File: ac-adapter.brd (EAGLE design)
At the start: 81.3 x 73.7 mm, 45 parts, among them IC2 TL431, Q1 300V5A, Q2 300V5A, Q3 TLP621-1, T1 COMMON_FILTER-SU10VFC, T2 TRANSFORMAER_FLYBACK-PQ2620, T3 COMMON_FILTER-SMALL

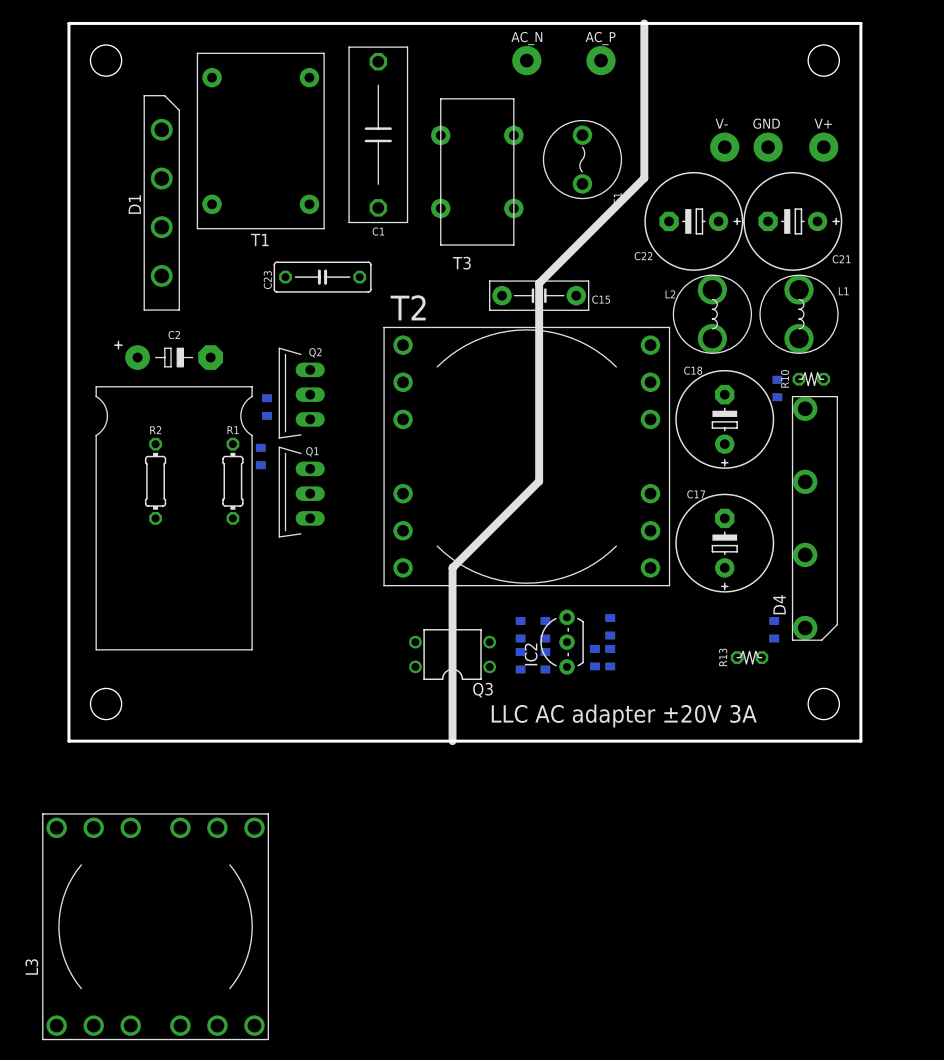
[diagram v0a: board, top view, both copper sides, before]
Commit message: 定数決まらん
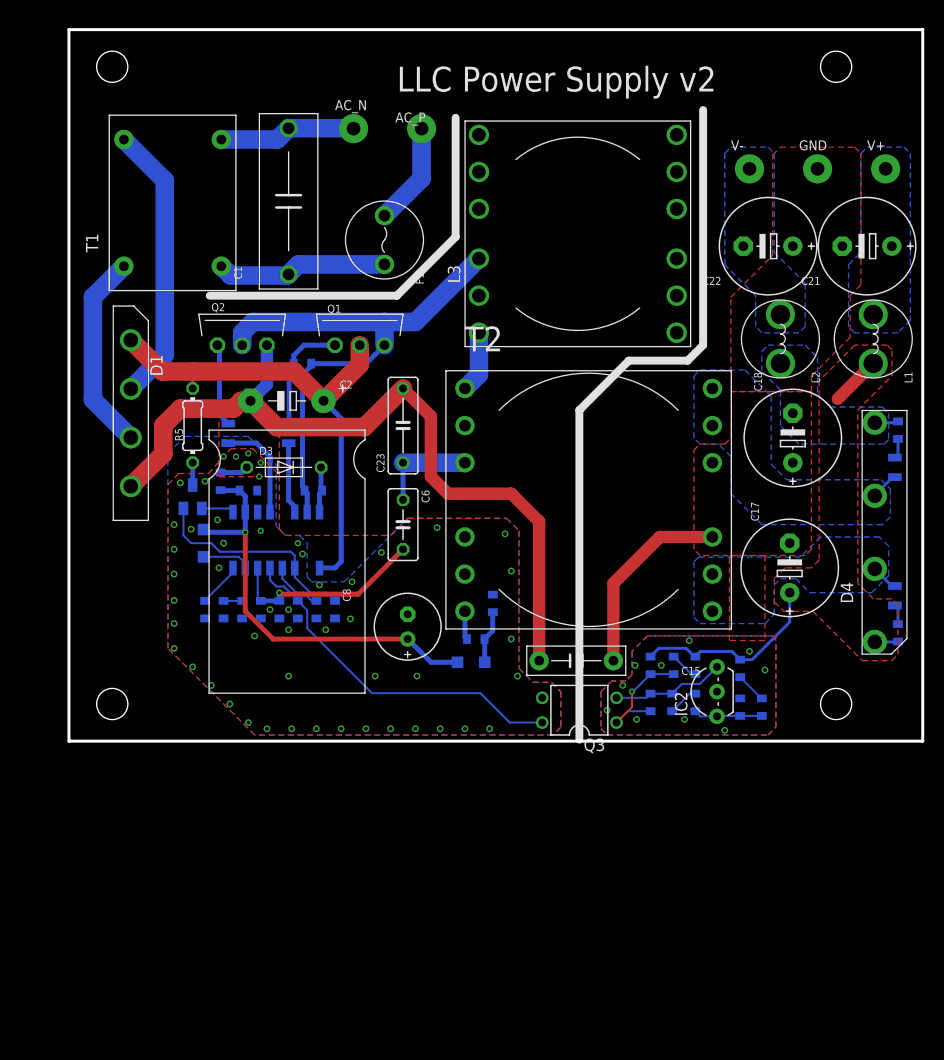
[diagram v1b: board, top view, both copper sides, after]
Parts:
- removed T3: COMMON_FILTER-SMALL, my_rcl:COMMON_FILTER__SMALL
- added C10, C3: 100p, my_rcl:1608
- added C11: 10000p, my_rcl:1608
- added C4, R3, R9: (no value), my_rcl:1608
- added C5, C7: 0.1u, my_rcl:1608
- added C6: 1kV 470p, my_rcl:C050
- added C8: 100u, my_rcl:E2.5-6.5
- added C9: 1000p, my_rcl:1608
- added D2: 100V0.1A, my_rcl:SOD123
- added D3: 600V1A, my_rcl:D0204/7
- added D6: 12V, my_rcl:SOD123
- added IC1: NCP13992, my_ic:SO16-NCP13992
- added Q4: BSS128, my_ic:SC59
- added R11, R4: 10, my_rcl:1608
- added R12: 1.5k, my_rcl:1608
- added R5: 1M, my_rcl:0204/7
- added R6, R7: 10k, my_rcl:1608
- added R8: 47k, my_rcl:1608
- C17, C18: value 1000u -> 470u
- C2: device my_rcl:E5-16A -> my_rcl:E5-16A2
- C24: value 0.1u -> 3300p
- Q1, Q2: value 300V5A -> 300V 5A
- R1, R2: value 22 -> 10; device my_rcl:0204/7 -> my_rcl:2012
- R10, R13: value 22 -> 10; device my_rcl:0207/2V -> my_rcl:2012
- R17: value 1.5k -> 5k
- moved L3 83.3 mm to (52.2, 52.1)
- moved C15 37.7 mm to (52.1, 8.26)
- moved F1 21.9 mm to (32.4, 51.4)
- moved D1 21.8 mm to (6.35, 33.7)
- moved TP1 19.7 mm to (36.2, 62.9)
- moved TP2 19.1 mm to (29.2, 62.9)
- moved C23 17.3 mm to (34.3, 32.4), turned to 90 degrees
- moved R15 16.4 mm to (71.1, 3.49)
- moved R13 16.2 mm to (84.8, 14.9), flipped to the bottom, turned to 90 degrees
- moved IC2 16.2 mm to (66.5, 5.08)
- moved Q1 16.1 mm to (29.8, 40.6), turned to 0 degrees
- moved C24 16.0 mm to (64.3, 3.97)
- moved R14 15.8 mm to (68.9, 3.49)
- moved R19 15.0 mm to (61.9, 3.97)
- moved Q3 14.2 mm to (52.4, 3.17)
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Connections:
- removed net N$30: T3.1, TP2.1
- removed net N$31: F1.2, T3.4
- removed net N$43: Q3.3
- removed net N$44: C2.-, C23.2, D1.4, Q2.3, R21.1
- new net N$12: IC1.8, R7.2
- new net N$13: C3.1, D6.1, IC1.7, R8.2
- new net N$14: C4.1, C6.2, IC1.6, R9.2
- new net N$15: IC1.4, R6.2
- new net N$16: IC1.14, R1.1
- new net N$17: IC1.12, R2.2
- new net N$18: C5.1, D3.2, IC1.16
- new net N$19: IC1.3, Q4.2, R3.2
- new net N$20: C10.1, IC1.5, Q3.4
- new net N$21: Q4.3, R5.1
- new net N$23: C11.1, R12.2
- new net N$24: C9.1, D2.1, R4.1
- new net N$25: D3.1, R11.2
- new net PFC_MODE: IC1.9, Q4.1
- new net PGND: C10.2, C15.2, C2.-, C23.2, C3.2, C4.2, C7.2, C8.-, C9.2, D1.4, IC1.11, Q2.3, Q3.3, R21.1, R3.1, R6.1, R7.1, R8.1, R9.1, T2.5
- new net VCC: C7.1, C8.+, D2.2, D6.2, IC1.10, R11.1
- net N$1: now also F1.2; no longer T3.3
- net N$11: no longer L3.4, L3.5
- net N$2: now also R1.2; no longer R1.1
- net N$22: now also R4.2, T2.6; no longer Q3.4
- net N$26: now also TP2.1; no longer T3.2
- net N$3: now also R13.1; no longer R13.2
- net N$34: now also R12.1
- net N$35: now also R13.2; no longer C19.2
- net N$40: now also C11.2, C19.2; no longer R13.1
- net N$8: now also C6.1
- net SW: now also C5.2, IC1.15, L3.4; no longer L3.1, L3.2, L3.3
- net VH: now also IC1.1, R5.2
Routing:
- net PGND: track 0.00 -> 83.1 mm, vias 0 -> 51
- net SW: track 0.00 -> 55.3 mm
- net VH: track 0.00 -> 51.1 mm
- net VCC: track 0.00 -> 43.0 mm, vias 0 -> 1
- net N$20: track 0.00 -> 36.4 mm
- net N$5: track 0.00 -> 28.8 mm
- net N$40: track 0.00 -> 27.7 mm
- net N$19: track 0.00 -> 22.4 mm
- net N$14: track 0.00 -> 21.2 mm, vias 0 -> 1
- net N$4: track 0.00 -> 20.5 mm
- net GND: track 0.00 -> 20.1 mm, vias 0 -> 10
- net N$1: track 0.00 -> 17.6 mm
- net N$26: track 0.00 -> 14.1 mm
- net N$34: track 0.00 -> 12.8 mm, vias 0 -> 1
- net N$2: track 0.00 -> 11.9 mm
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- added copper zone on layer 1, net GND
- added copper zone on layer 16, net GND
- added copper zone on layer 16, net N$35
- added copper zone on layer 16, net N$36
- added copper zone on layer 1, net N$40
- added copper zone on layer 16, net N$7
- added copper zone on layer 1, net PGND
- added copper zone on layer 16, net PGND
- added copper zone on layer 16, net V+
- added copper zone on layer 16, net V-
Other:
- board size 81.3 x 73.7 mm -> 87.6 x 73 mm
- board text added: "LLC Power Supply v2"
- board text removed: "LLC AC adapter ±20V 3A"
